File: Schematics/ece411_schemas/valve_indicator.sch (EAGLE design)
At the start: 68 parts, among them IC1 STM32F042K6T6, T1 2N2222, T2 2N2222, T3 2N2222, T4 2N2222, U1 DIODES_INC._AZ34063UMTR-G1DIO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, U2 DIODES_INC._AZ34063UMTR-G1DIO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

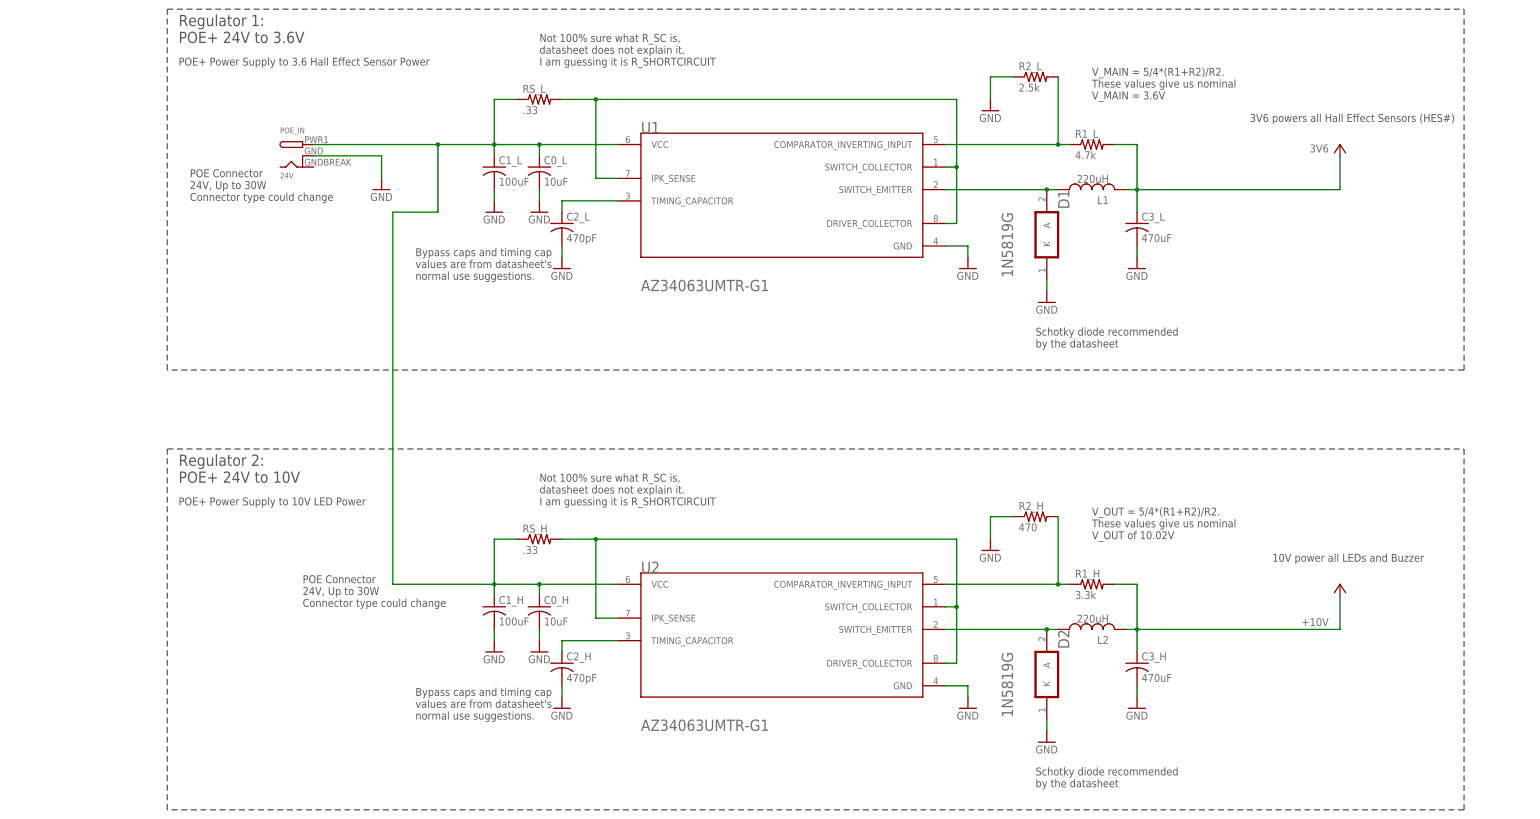
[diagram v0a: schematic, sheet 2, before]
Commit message: added bat backup
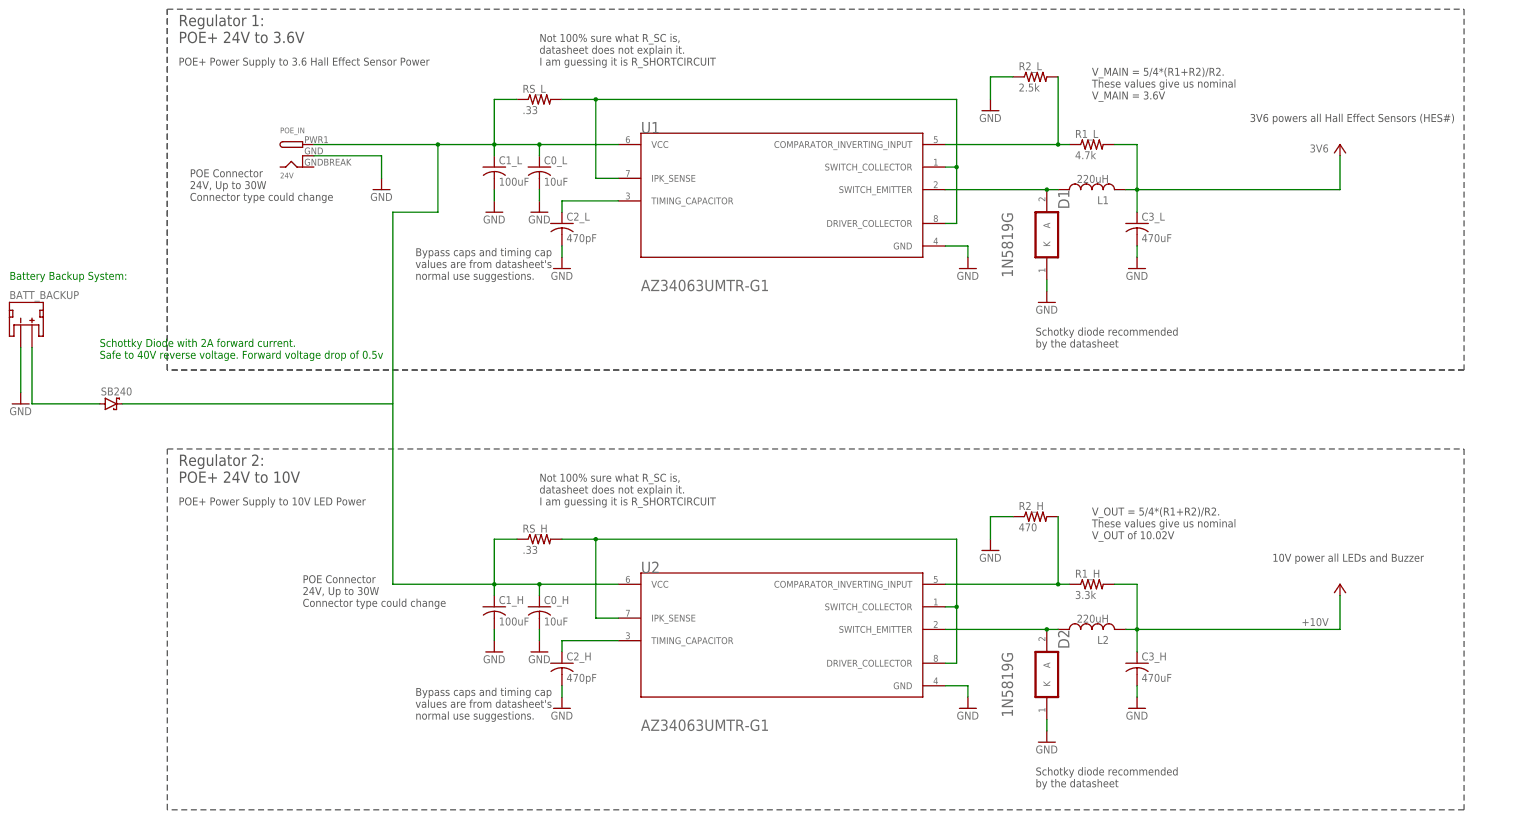
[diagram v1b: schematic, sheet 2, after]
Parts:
- added BATT_BACKUP: (no value), SparkFun-Connectors:JST_2MM_MALE
- added SB240: (no value), diode:SCHOTTKY-DIODECB417-15
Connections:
- new net N$10: SB240.C
- new net N$16: BATT_BACKUP.+, SB240.A
- net GND: now also BATT_BACKUP.-
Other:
- note added: "Battery Backup System:"
- note added: "Schottky Diode with 2A forward current. Safe to 40V reverse voltage. Forward voltage drop of 0.5v"
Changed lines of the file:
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@@
 <part name="GND41" library="supply1" library_urn="urn:adsk.eagle:library:371" deviceset="GND" device=""/>
 <part name="GND42" library="supply1" library_urn="urn:adsk.eagle:library:371" deviceset="GND" device=""/>
+<part name="BATT_BACKUP" library="SparkFun-Connectors" library_urn="urn:adsk.eagle:library:513" deviceset="JST_2MM_MALE" device="" package3d_urn="urn:adsk.eagle:package:38042/1"/>
+<part name="GND43" library="supply1" library_urn="urn:adsk.eagle:library:371" deviceset="GND" device=""/>
+<part name="SB240" library="diode" library_urn="urn:adsk.eagle:library:210" deviceset="SCHOTTKY-DIODE" device="CB417-15" package3d_urn="urn:adsk.eagle:package:43349/2"/>
 </parts>
 <sheets>
@@
 <text x="297.18" y="119.38" size="1.778" layer="97">10V power all LEDs and Buzzer</text>
 <text x="50.8" y="132.08" size="1.778" layer="97">POE+ Power Supply to 10V LED Power</text>
+<wire x1="340.36" y1="162.56" x2="48.26" y2="162.56" width="0.1524" layer="97" style="shortdash"/>
+<wire x1="48.26" y1="162.56" x2="48.26" y2="243.84" width="0.1524" layer="97" style="shortdash"/>
+<text x="12.7" y="182.88" size="1.778" layer="91">Battery Backup System:</text>
+<text x="33.02" y="165.1" size="1.778" layer="91">Schottky Diode with 2A forward current.
+Safe to 40V reverse voltage. Forward voltage drop of 0.5v</text>
 </plain>
 <instances>
@@
 <attribute name="VALUE" x="129.54" y="195.58" size="1.778" layer="96"/>
 </instance>
+<instance part="BATT_BACKUP" gate="G$1" x="15.24" y="172.72" smashed="yes">
+<attribute name="NAME" x="12.7" y="178.562" size="1.778" layer="95"/>
+</instance>
+<instance part="GND43" gate="1" x="15.24" y="154.94" smashed="yes">
+<attribute name="VALUE" x="12.7" y="152.4" size="1.778" layer="96"/>
+</instance>
+<instance part="SB240" gate="G$1" x="35.56" y="154.94" smashed="yes">
+<attribute name="NAME" x="33.274" y="156.845" size="1.778" layer="95"/>
+<attribute name="VALUE" x="33.274" y="151.511" size="1.778" layer="96"/>
+</instance>
 </instances>
 <busses>
@@
 <pinref part="C0_L" gate="G$1" pin="2"/>
 <wire x1="132.08" y1="200.66" x2="132.08" y2="203.2" width="0.1524" layer="91"/>
+</segment>
+<segment>
+<pinref part="BATT_BACKUP" gate="G$1" pin="-"/>
+<pinref part="GND43" gate="1" pin="GND"/>
+<wire x1="15.24" y1="167.64" x2="15.24" y2="157.48" width="0.1524" layer="91"/>
 </segment>
 </net>
@@
 </segment>
 </net>
+<net name="N$10" class="0">
+<segment>
+<pinref part="SB240" gate="G$1" pin="C"/>
+<wire x1="38.1" y1="154.94" x2="99.06" y2="154.94" width="0.1524" layer="91"/>
+</segment>
+</net>
+<net name="N$16" class="0">
+<segment>
+<pinref part="BATT_BACKUP" gate="G$1" pin="+"/>
+<pinref part="SB240" gate="G$1" pin="A"/>
+<wire x1="17.78" y1="167.64" x2="17.78" y2="154.94" width="0.1524" layer="91"/>
+<wire x1="17.78" y1="154.94" x2="33.02" y2="154.94" width="0.1524" layer="91"/>
+</segment>
+</net>
